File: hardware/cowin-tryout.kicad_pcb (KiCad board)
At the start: 2 copper layers, 63 x 58 mm, 94 parts, among them J1 BMP180_HEADER, J10 USB_DBG, J2 CONN_PMS, J3 SHT3x_HEADER, J7 DEBUG_HEADER, J8 BAT, J9 DHT22_HEADER, Q1 SS9013_J3, Q2 SS9013_J3, SW1 FLASH_BUTTON, SW2 SW_RESET,2_leg,SMD, U1 BMP180, U10 SSD1306-OLED-I2C, U11 AMS1117-3.3, U12 DESIGNED_IN_HONG_KONG, U13 GITHUB_ADDRESS, U14 TTL_TERMINAL, U15 BOARD_REVISION, U16 MCP73831, U17 24C02_SOIC8, U2 ML8511, U3 PMS5003S_BODY, U4 SHT3x-DIS, U5 74AHCT1G125, U6 ESP12, U7 CH340T, U8 USB_Micro, U9 SSD1306-OLED-I2C, Y1 O_12M,3225

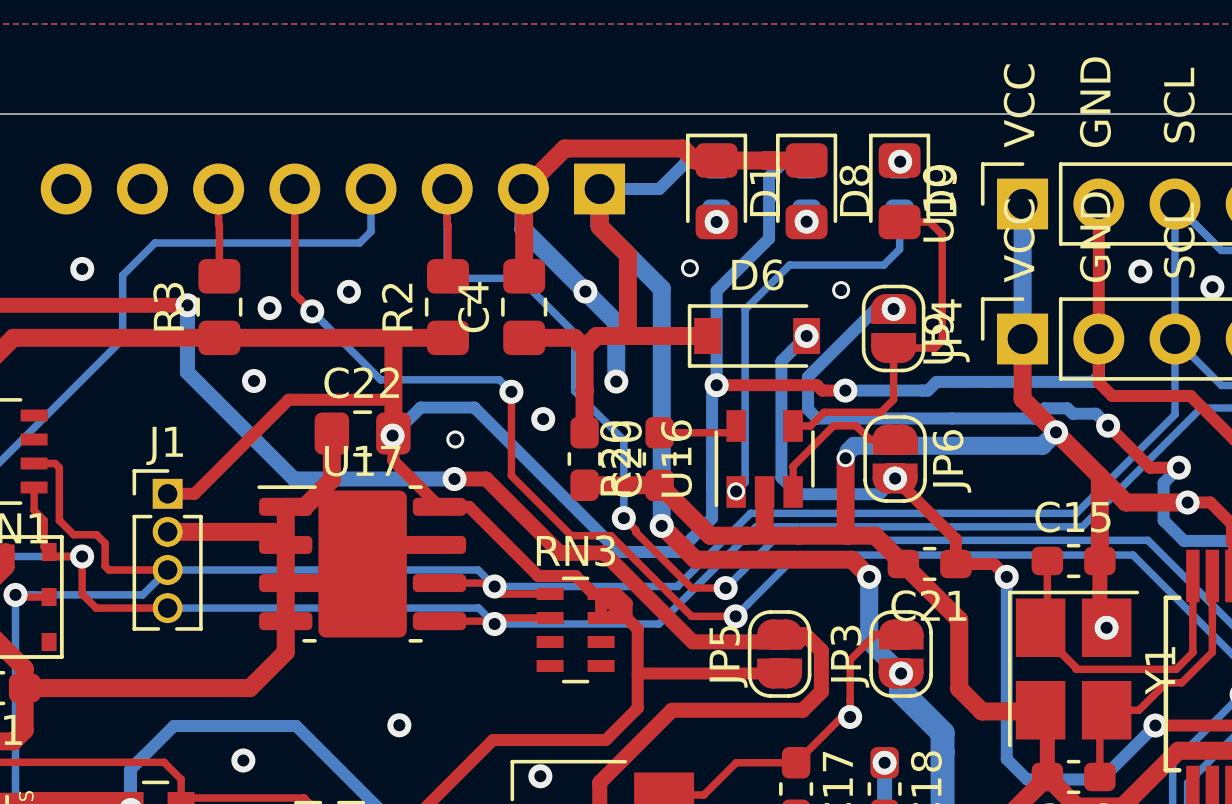
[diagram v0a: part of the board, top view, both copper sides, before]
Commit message: update,
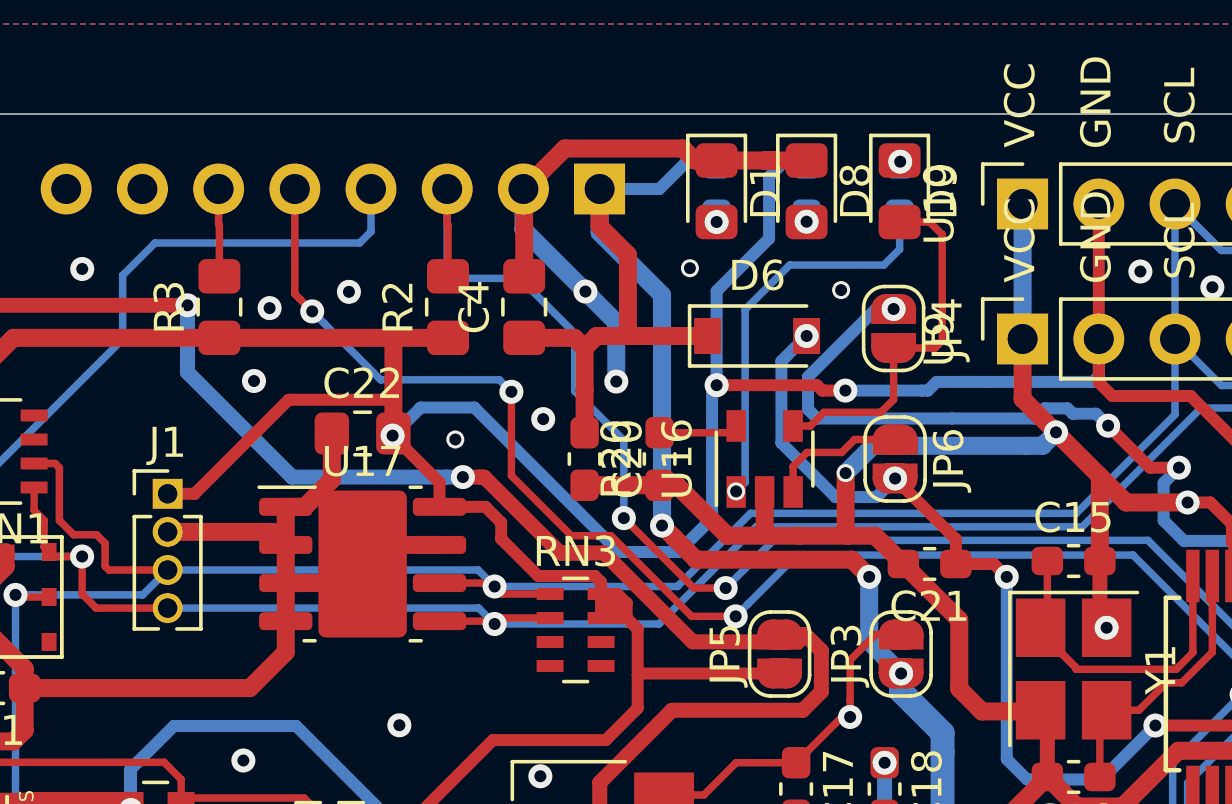
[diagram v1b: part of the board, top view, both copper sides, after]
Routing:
- net +3V3: track 300.7 -> 302.4 mm
- net Vbat: track 40.7 -> 40.1 mm
